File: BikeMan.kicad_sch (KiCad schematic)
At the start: 20 parts, among them J10 USB_A_stacked, J11 PushConnector_8pos, J13 USB_A_stacked, J14 PushConnector_8pos, J2 Conn_01x06_Male, J3 Conn_01x06_Male, J4 Conn_01x06_Female, J7 PushConnector_8pos, J8 Conn_01x06_Female, J9 Conn_01x06_Female, Q5 DMN62D0U-7, Q6 DMN62D0U-7

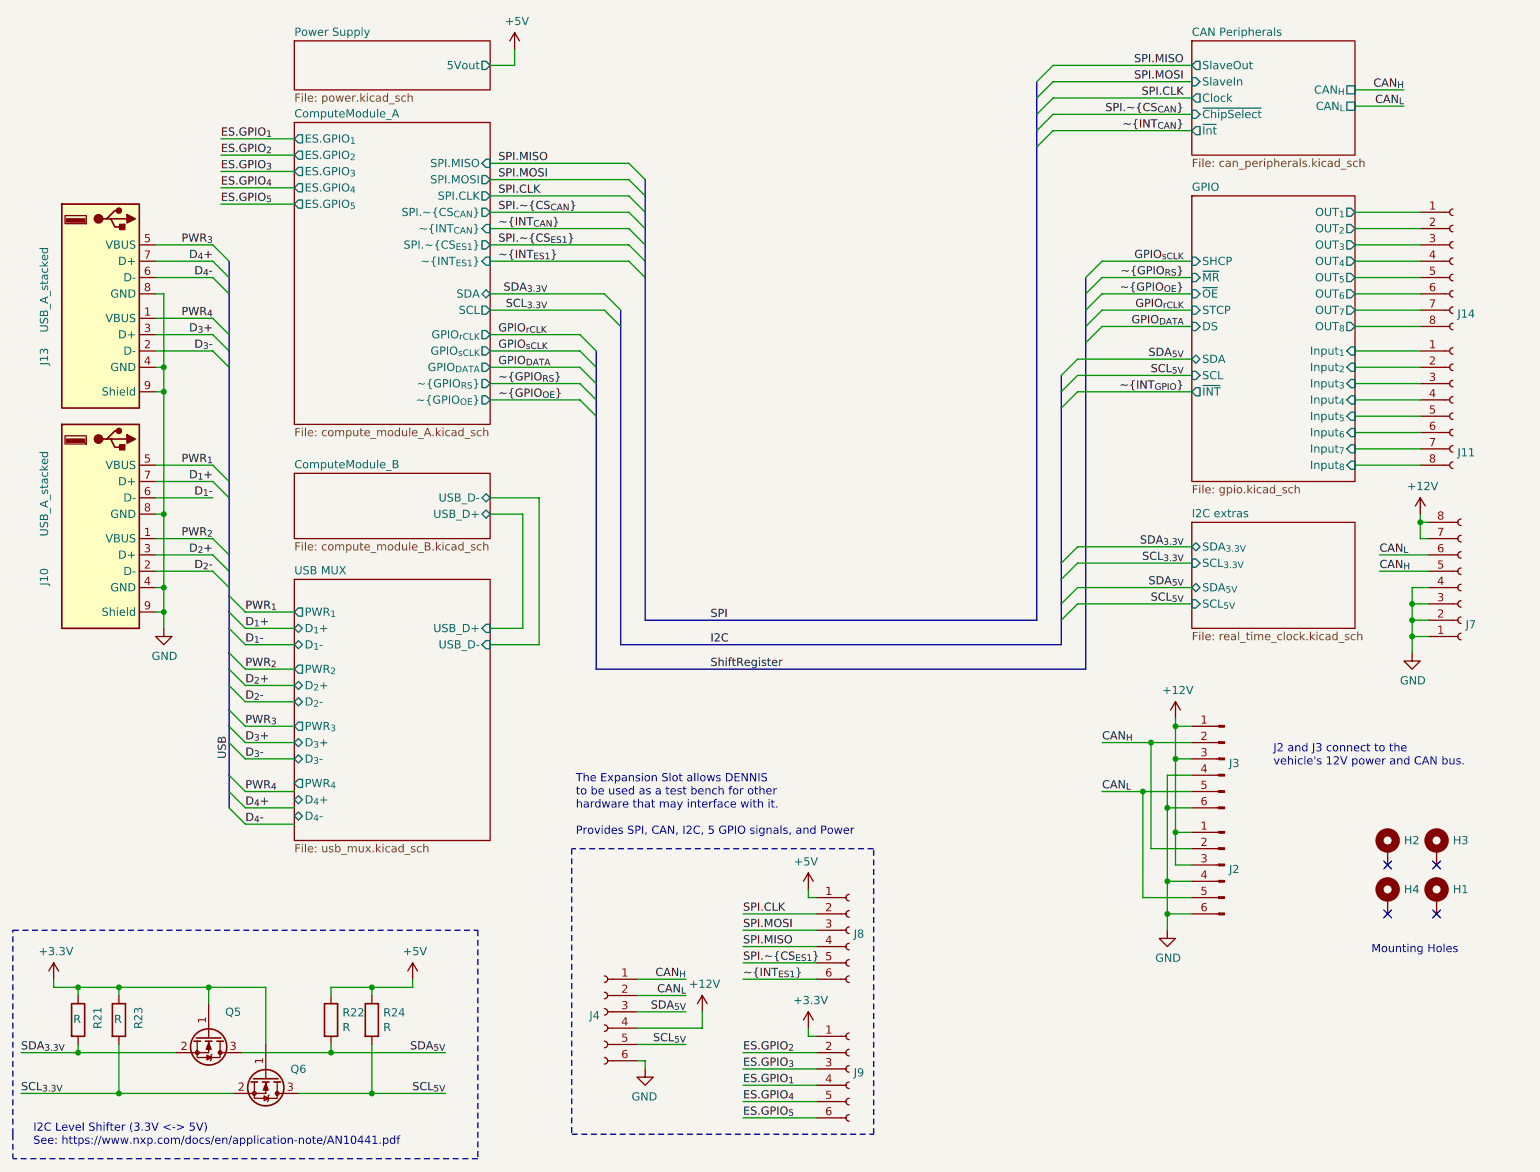
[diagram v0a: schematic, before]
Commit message: migrated computers
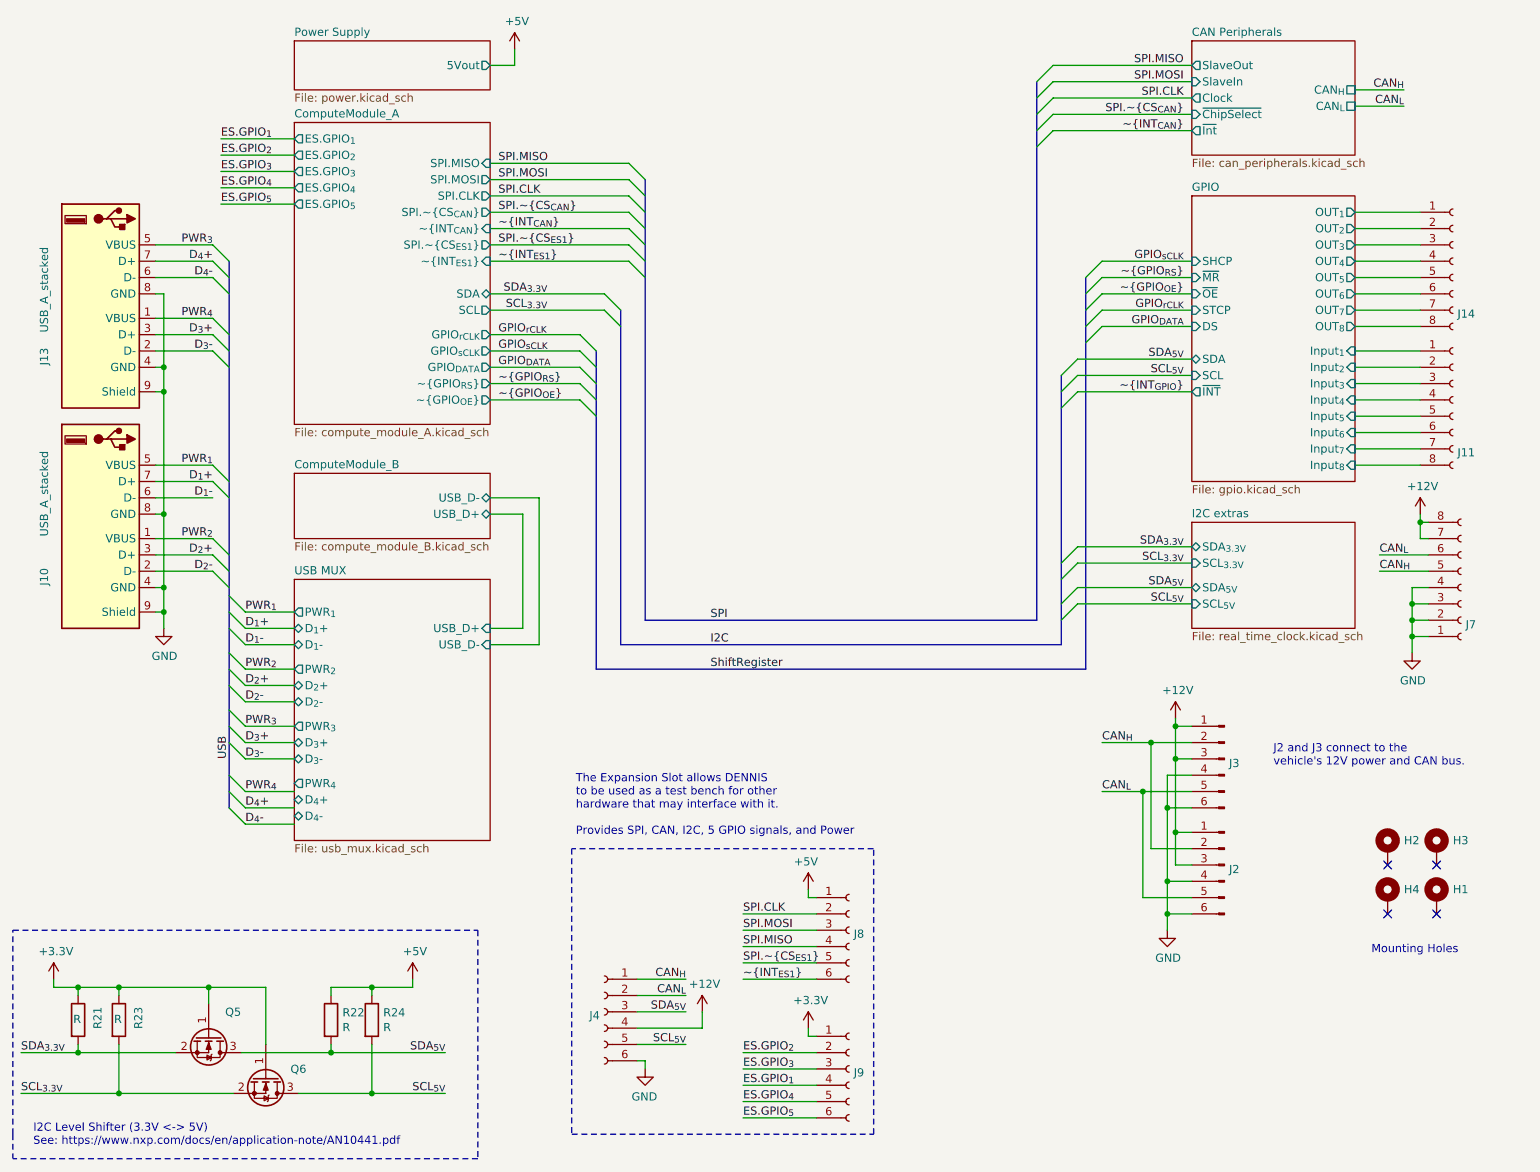
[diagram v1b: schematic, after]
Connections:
- net SPI.~CS_{ES1} renamed SPI.~{CS_{ES1}}
- net ~INT_{ES1} renamed ~{INT_{ES1}}
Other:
- sheet CAN Peripherals ports: added ~{ChipSelect}, ~{Int}; removed ~ChipSelect, ~Int
- sheet ComputeModule_A ports: added SPI.~{CS_{CAN}}, SPI.~{CS_{ES1}}, ~{GPIO_{OE}}, ~{GPIO_{RS}}, ~{INT_{CAN}}, ~{INT_{ES1}}; removed SPI.~CS_{CAN}, SPI.~CS_{ES1}, ~GPIO_{OE}, ~GPIO_{RS}, ~INT_{CAN}, ~INT_{ES1}
- sheet GPIO ports: added ~{INT}, ~{MR}, ~{OE}; removed ~INT, ~MR, ~OE
